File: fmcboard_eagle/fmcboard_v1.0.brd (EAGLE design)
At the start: 98 x 74 mm, 39 parts, among them IC1 OPA699ID, IC2 OPA699ID, IC3 ICL7660CPA, IC4 ICL7660CPA, J1 8pin, J12 4p-2.54, J2 ASP-134604-01, J3 4p-2.54, J4 4p-2.54, J5 8pin, U1 TXS0108EPWR-TSSOP20

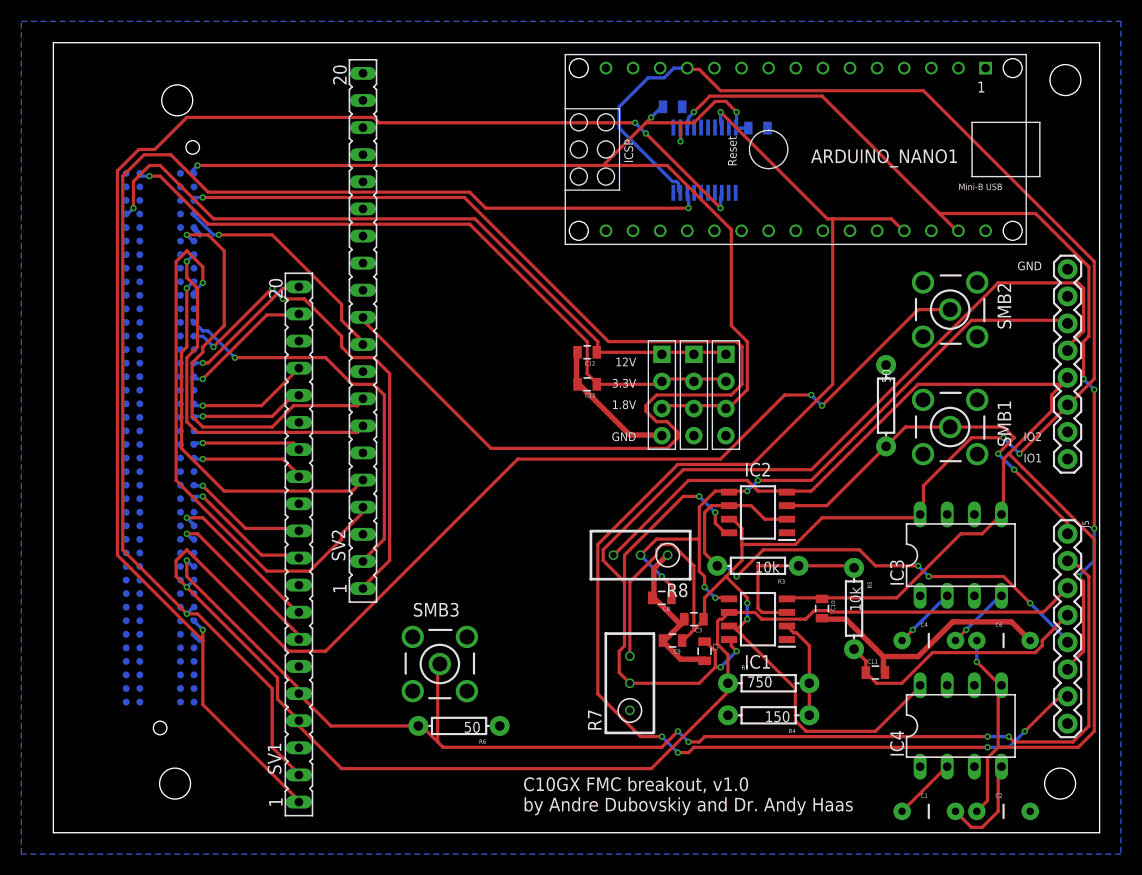
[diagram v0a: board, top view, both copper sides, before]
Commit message: fmcboard v1 submitted
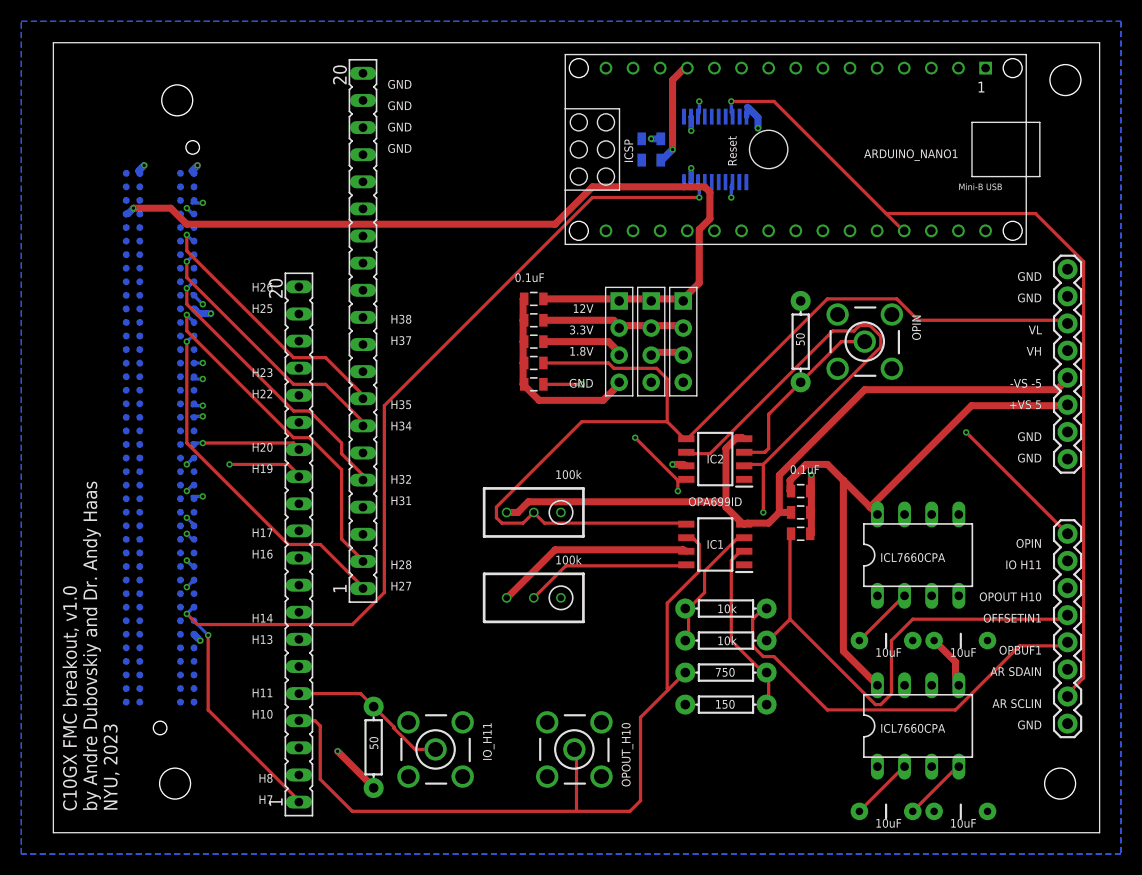
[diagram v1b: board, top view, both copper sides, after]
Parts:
- removed SMB1, SMB2, SMB3: BU-SMB-V, con-coax:BU-SMB-V
- added IO_H11, OPIN, OPOUT_H10: BU-SMB-V, con-coax:BU-SMB-V
- U1: value TXS0108EPWR-TSSOP20 -> TXS0108EPWR
- moved C9 45.0 mm to (56.0, 63.0), flipped to the bottom, turned to 0 degrees
- moved C7 29.7 mm to (45.0, 42.0), turned to 180 degrees
- moved C5 29.0 mm to (45.0, 46.0), flipped to the top
- moved C8 25.1 mm to (45.0, 44.0)
- moved C3 15.6 mm to (70.0, 32.0), turned to 0 degrees
- moved C11 14.8 mm to (70.0, 28.0)
- moved R5 12.4 mm to (63.0, 18.0), turned to 0 degrees
- moved R7 12.0 mm to (45.0, 22.0), turned to 90 degrees
- moved R8 10.8 mm to (45.0, 30.0)
- moved R2 10.0 mm to (70.0, 46.0)
- moved C10 9.22 mm to (70.0, 30.0), turned to 0 degrees
- moved R6 8.25 mm to (30.0, 8.00), turned to 90 degrees
- moved IC1 8.06 mm to (62.0, 27.0)
- moved C13 7.81 mm to (45.0, 48.0)
- moved C12 7.07 mm to (45.0, 50.0)
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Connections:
- net GND: now also IO_H11.2, IO_H11.3, IO_H11.4, IO_H11.5, OPIN.2, OPIN.3, OPIN.4, OPIN.5, OPOUT_H10.2, OPOUT_H10.3, OPOUT_H10.4, OPOUT_H10.5; no longer SMB1.2, SMB1.3, SMB1.4, SMB1.5, SMB2.2, SMB2.3, SMB2.4, SMB2.5, SMB3.2, SMB3.3, SMB3.4, SMB3.5
- net IO1: now also OPIN.1; no longer SMB1.1
- net IO2_H11: now also IO_H11.1; no longer SMB3.1
- net OPOUT1_H10: now also OPOUT_H10.1; no longer SMB2.1
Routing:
- net H38: track 110.9 -> 20.9 mm
- net OPOUT1_H10: track 198.7 -> 131.9 mm, vias 3 -> 1
- net AR_SCLIN: track 129.6 -> 84.4 mm, vias 5 -> 1
- net GND: track 56.5 -> 100.3 mm, vias 0 -> 4
- net OPBUF1: track 51.9 -> 94.9 mm, vias 4 -> 1
- net VL: track 64.0 -> 100.0 mm, vias 5 -> 0
- net SDAIN: track 121.8 -> 97.0 mm
- net SCLIN: track 132.4 -> 108.6 mm, vias 4 -> 2
- net -VS: track 146.0 -> 123.0 mm, vias 1 -> 0
- net OFFSETIN1: track 24.9 -> 47.1 mm
- net IO2_H11: track 120.1 -> 99.5 mm, vias 5 -> 1
- net H31: track 51.3 -> 32.1 mm
- net H35: track 39.4 -> 24.8 mm
- net VH: track 108.3 -> 94.4 mm, vias 4 -> 3
- net 12V: track 68.0 -> 81.9 mm
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- added copper zone on layer 2, net GND
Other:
- board outline removed
- board text added: "+VS 5"
- board text added: "-VS -5"
- board text added: "AR SCLIN"
- board text added: "AR SDAIN"
- board text added: "C10GX FMC breakout, v1.0 by Andre Dubovskiy and Dr. Andy Haas NYU, 2023"
- board text added: "H10"
- board text added: "H11"
- board text added: "H13"
- board text added: "H14"
- board text added: "H16"
- board text added: "H17"
- board text added: "H19"
- board text added: "H20"
- board text added: "H22"
- board text added: "H23"
- board text added: "H25"
- board text added: "H26"
- board text added: "H27"
- board text added: "H28"
- board text added: "H31"
- board text added: "H32"
- board text added: "H34"
- board text added: "H35"
- board text added: "H37"
- board text added: "H38"
- board text added: "H7"
- board text added: "H8"
- board text added: "IO H11"
- board text added: "OFFSETIN1"
- board text added: "OPBUF1"
- board text added: "OPIN"
- board text added: "OPOUT H10"
- board text added: "VH"
- board text added: "VL"
- board text removed: "C10GX FMC breakout, v1.0 by Andre Dubovskiy and Dr. Andy Haas"
- board text removed: "IO1"
- board text removed: "IO2"
